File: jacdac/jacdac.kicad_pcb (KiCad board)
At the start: 2 copper layers, 62.9 x 33.4 mm, 12 parts, among them J1 Meow Conec2, J2 Meow Conec1, J3 Audio_Jack_TRRS, J4 Audio_Jack_TRRS, J5 Audio_Jack_TRRS, J6 Audio_Jack_TRRS

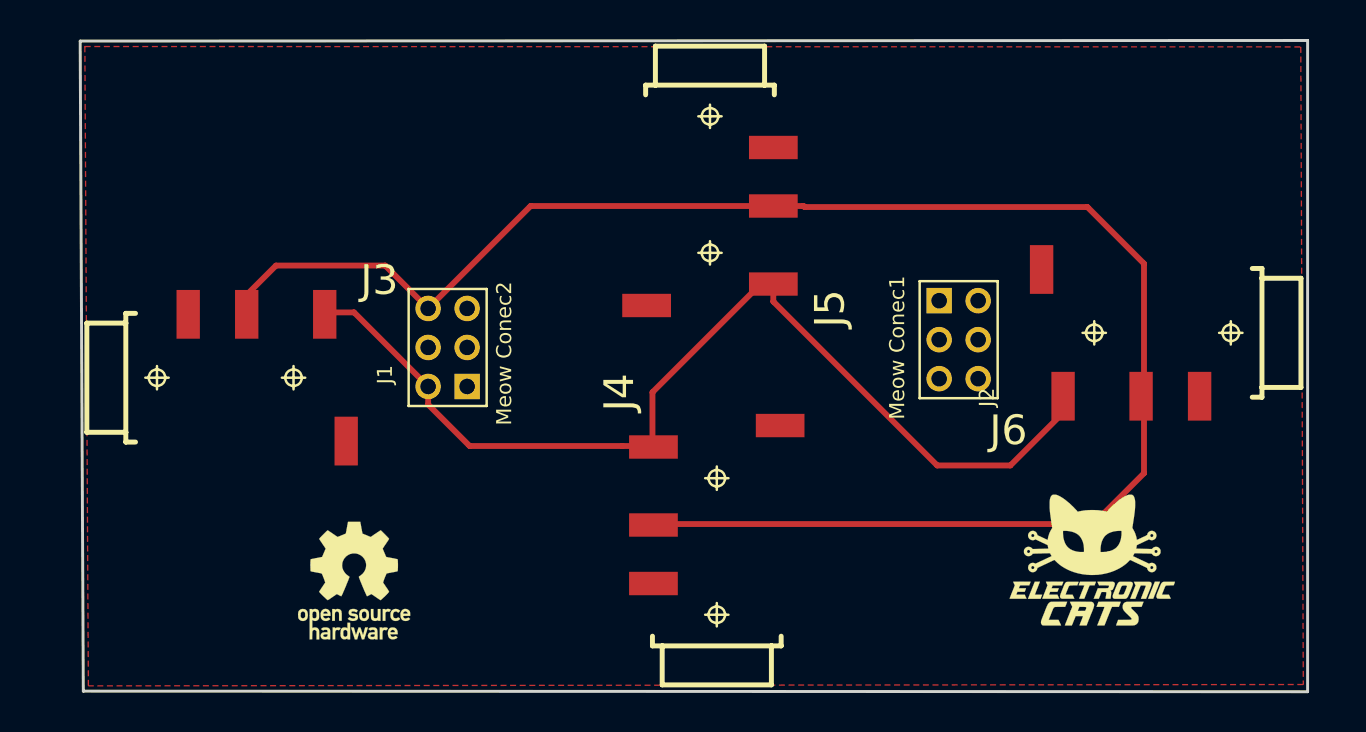
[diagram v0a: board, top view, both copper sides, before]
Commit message: update PCB
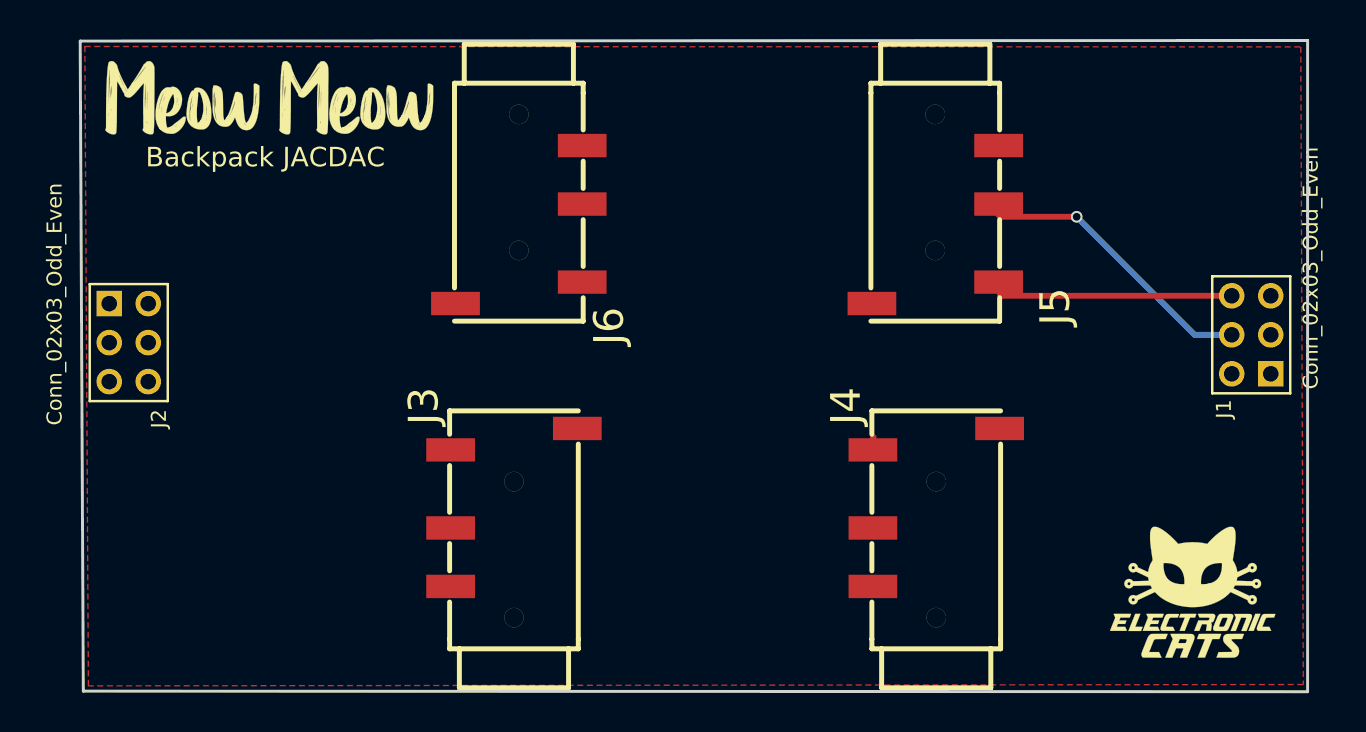
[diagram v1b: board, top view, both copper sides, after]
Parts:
- added G***: LOGO, LOGO, F.Cu at (87.3, 38.9)
- added G***: LOGO, LOGO, B.Cu at (124.3, 39.6)
- J1: value Meow Conec2 -> Conn_02x03_Odd_Even
- J2: value Meow Conec1 -> Conn_02x03_Odd_Even
- REF***: moved to B.Cu
- moved REF*** 58.2 mm to (136.9, 64.2)
- moved J2 42.6 mm to (80.1, 51.4)
- moved REF*** 42.5 mm to (129.2, 64.0)
- moved J1 41.2 mm to (137.7, 51.0)
- moved J6 40.2 mm to (100.1, 38.0), turned to 270 degrees
- moved REF*** 33.0 mm to (118.3, 64.1)
- moved J3 24.3 mm to (99.8, 67.0), turned to 90 degrees
- moved REF*** 17.6 mm to (109.2, 64.2), turned to 180 degrees
- moved G*** 12.2 mm to (86.1, 62.5)
- moved J5 11.6 mm to (121.5, 38.0)
- moved J4 11.3 mm to (121.5, 67.0)
- moved G*** 5.41 mm to (134.7, 64.2)
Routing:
- net /JACDAC_TX: track 89.0 -> 15.1 mm, vias 0 -> 1
- net VCC: track 52.9 -> 12.0 mm
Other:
- board text added: "Backpack JACDAC"
- board text added: "JACDAC - Connect with audio cable 3.5mm"
- board text removed: "JACDAC - Connect with cable 3.5mm"
- board text removed: "Meow Meow Backpack JACDAC"
